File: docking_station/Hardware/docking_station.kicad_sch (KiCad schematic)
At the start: 26 parts, among them IC1 VOM1271T, IC2 VOM1271T, J1 SUPPLY_EN, J2 LIVE_IN, J5 SUPPLY+, J6 SUPPLY-, K1 Fujitsu_FTR-LYCA005x, K2 EC2-3NU, K3 EC2-3NU, Q1 NMOS, Q2 NMOS, Q3 NMOS, Q4 NMOS, Q5 NMOS, Q6 NMOS, Q7 NMOS, Q8 NMOS, Q9 NMOS, U1 LTC4357MS8

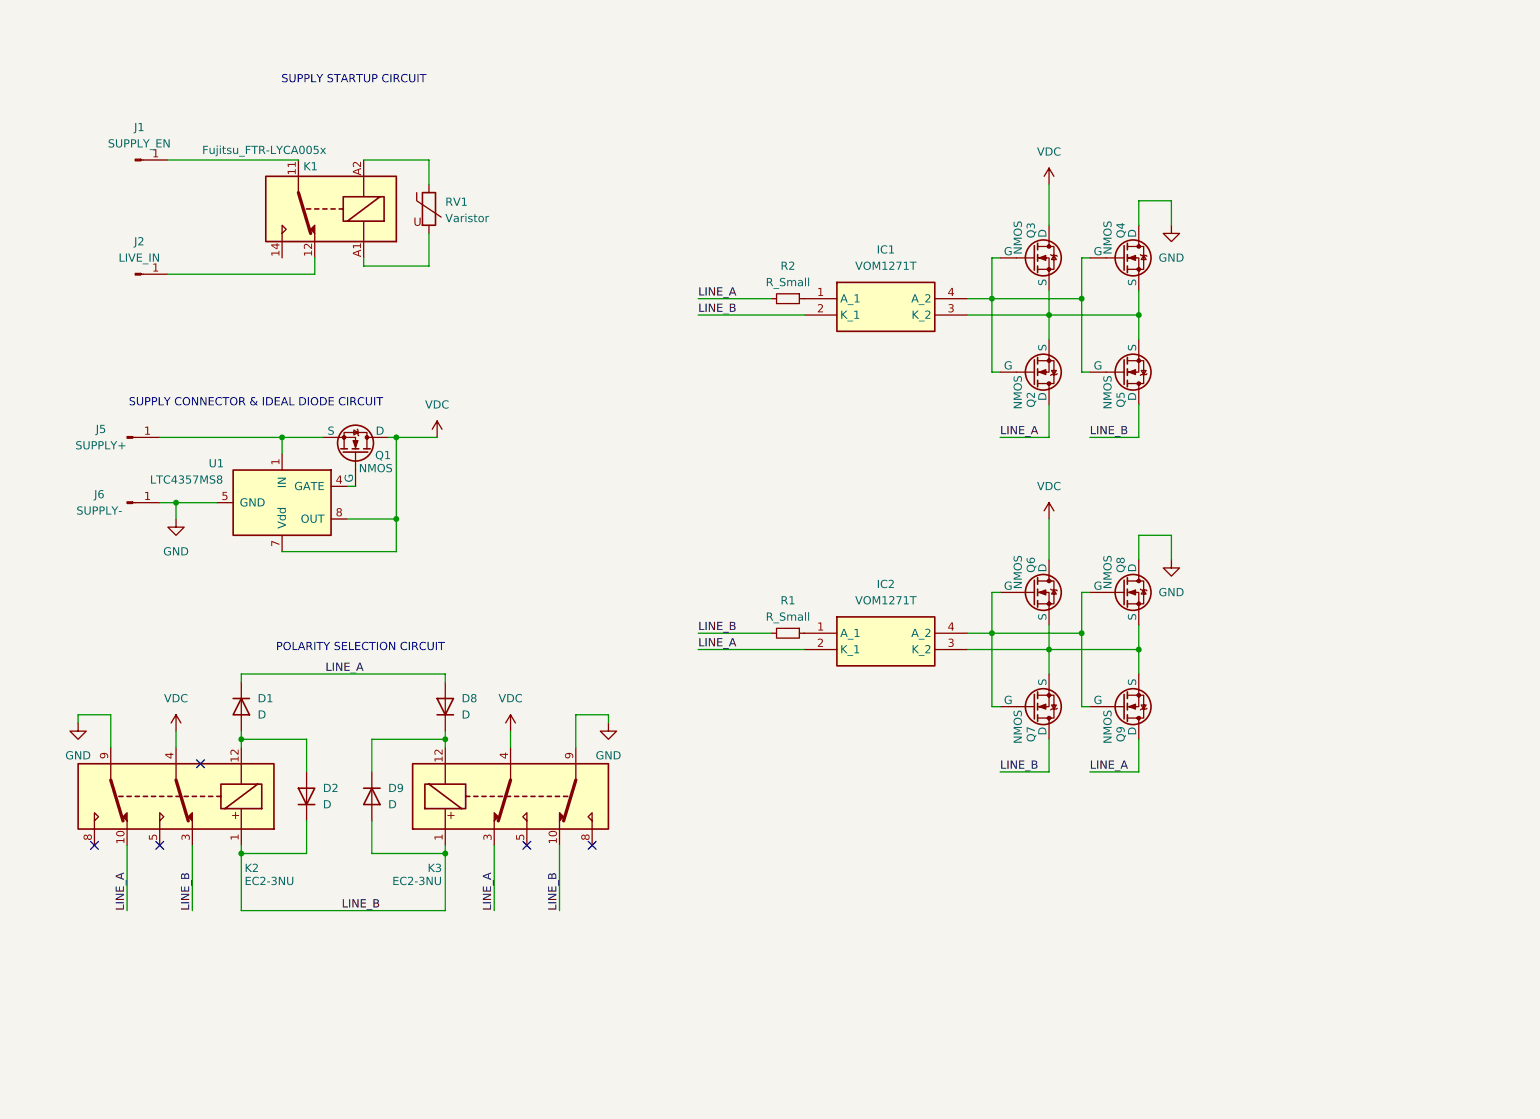
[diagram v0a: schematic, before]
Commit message: docking_station draft finished
a lot to do still - mostly calculation and review, but the bulk is done and I'm happy
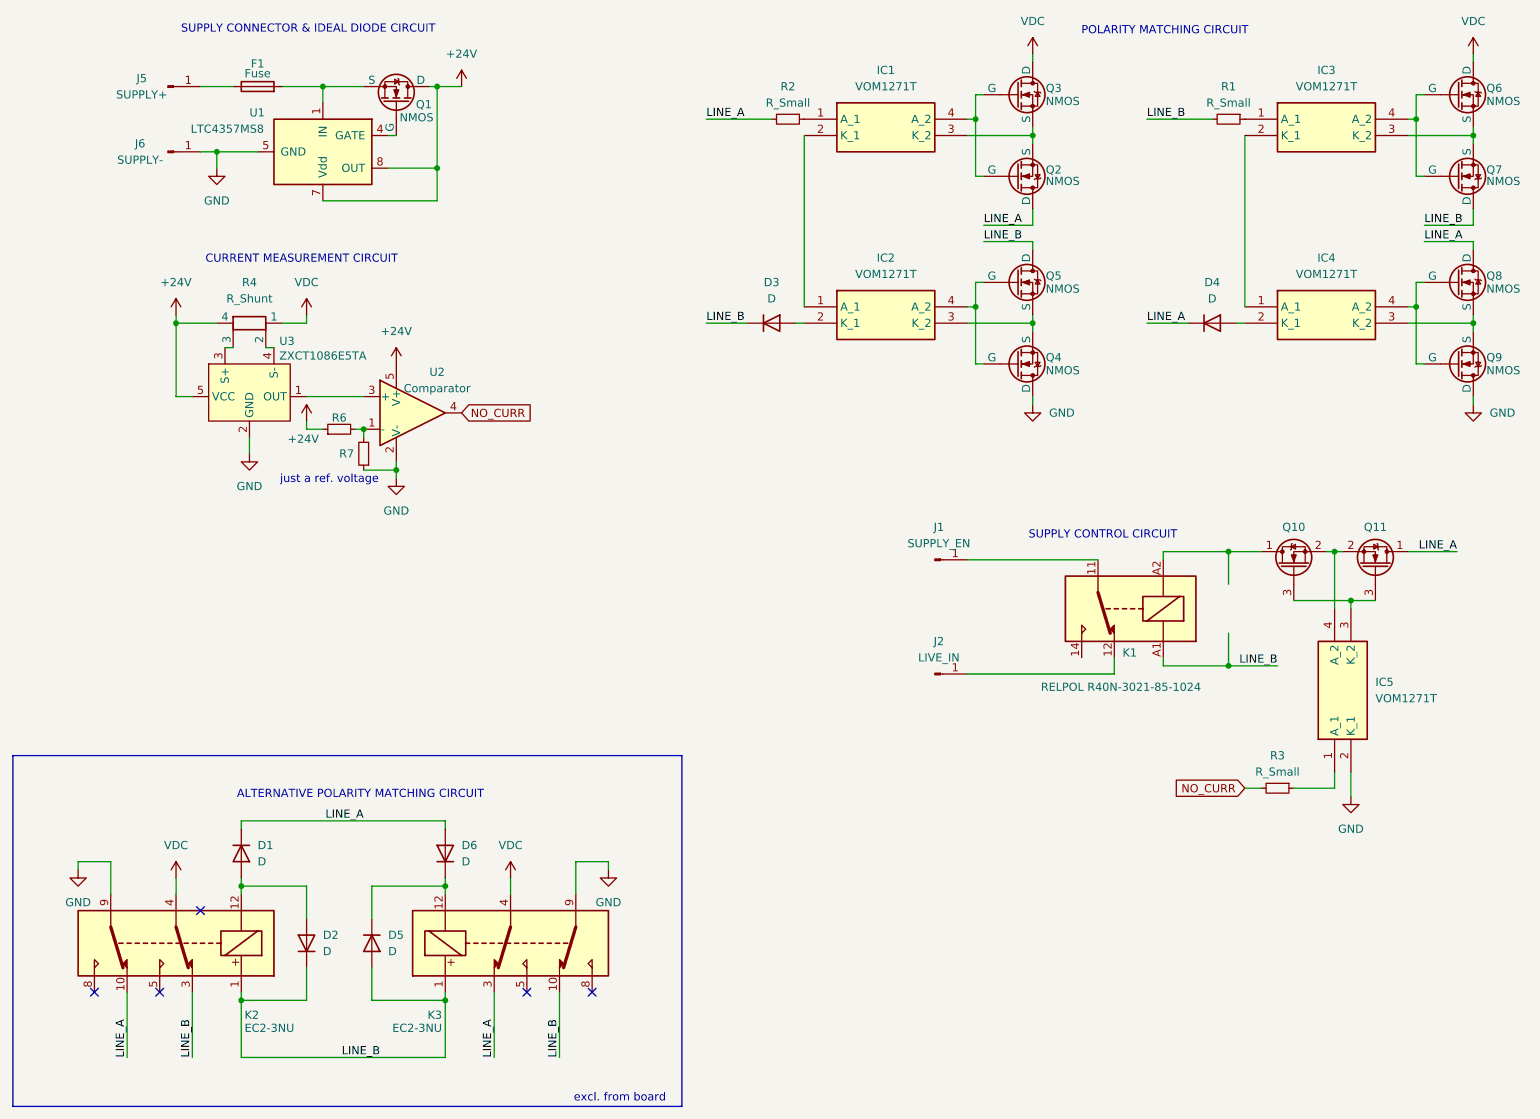
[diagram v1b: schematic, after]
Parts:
- removed D8, D9: D, symbol Device:D
- removed RV1: Varistor, symbol Device:Varistor
- added D3, D4, D5, D6: D, symbol Device:D
- added F1: Fuse, symbol Device:Fuse
- added IC3, IC4, IC5: VOM1271T, SOP254P675X240-4N, symbol VOM1271T:VOM1271T
- added Q10, Q11: Q_NMOS_Depletion_DSG, symbol Device:Q_NMOS_Depletion_DSG
- added R3, R6, R7: R_Small, symbol Device:R_Small
- added R4: R_Shunt, symbol Device:R_Shunt
- added U2: Comparator, Package_TO_SOT_SMD:SOT-23-5, symbol Comparator:LM397
- added U3: ZXCT1086E5TA, Package_TO_SOT_SMD:SOT-23-5, symbol FIRO_collected:ZXCT1086E5TA
- K1: value Fujitsu_FTR-LYCA005x -> RELPOL R40N-3021-85-1024
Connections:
- net GND: now also Q9.1 (D), IC5.2 (K_1), R7.1, U2.2 (V-), U3.2 (GND); no longer Q8.1 (D)
- net LINE_A: now also Q8.1 (D), D4.1 (K), D6.2 (A), Q11.1 (D); no longer IC2.2 (K_1), Q9.1 (D)
- net LINE_B: now also K1.A1, D3.1 (K), D5.2 (A); no longer IC1.2 (K_1)
- net VDC: now also R4.1; no longer Q1.1 (D), U1.7 (Vdd), U1.8 (OUT)
- net at K3.12: now also D5.1 (K), D6.1 (K)
- net at IC1.4 (A_2), Q2.2 (G), Q3.2 (G): no longer Q4.2 (G), Q5.2 (G)
- net at IC1.3 (K_2), Q2.3 (S), Q3.3 (S): no longer Q4.3 (S), Q5.3 (S)
- net at K1.A2: now also Q10.1 (D)
- net at Q1.3 (S), U1.1 (IN): now also F1.2; no longer J5.1 (Pin_1)
- net at R1.1: now also IC3.1 (A_1); no longer IC2.1 (A_1)
- new net: IC3.2 (K_1), IC4.1 (A_1)
- new net: IC3.3 (K_2), Q6.3 (S), Q7.3 (S)
- new net: IC3.4 (A_2), Q6.2 (G), Q7.2 (G)
- new net: F1.1, J5.1 (Pin_1)
- new net: IC5.4 (A_2), Q10.2 (S), Q11.2 (S)
- new net: IC5.3 (K_2), Q10.3 (G), Q11.3 (G)
- new net: IC5.1 (A_1), R3.1
- new net: IC4.4 (A_2), Q8.2 (G), Q9.2 (G)
- new net: IC4.3 (K_2), Q8.3 (S), Q9.3 (S)
- new net: R6.2, R7.2, U2.1 (-)
- new net: IC1.2 (K_1), IC2.1 (A_1)
- new net: IC2.4 (A_2), Q4.2 (G), Q5.2 (G)
- new net: IC2.3 (K_2), Q4.3 (S), Q5.3 (S)
- new net: D3.2 (A), IC2.2 (K_1)
- new net: U2.3 (+), U3.1 (OUT)
- new net: R4.3, U3.3 (S+)
- new net: R4.2, U3.4 (S-)
- new net: D4.2 (A), IC4.2 (K_1)
- new net +24V: Q1.1 (D), R4.4, R6.1, U1.7 (Vdd), U1.8 (OUT), U2.5 (V+), U3.5 (VCC)
- new net NO_CURR: R3.2, U2.4
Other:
- note added: "ALTERNATIVE POLARITY MATCHING CIRCUIT"
- note added: "CURRENT MEASUREMENT CIRCUIT"
- note added: "POLARITY MATCHING CIRCUIT"
- note added: "SUPPLY CONTROL CIRCUIT"
- note added: "excl. from board"
- note added: "just a ref. voltage"
- note removed: "POLARITY SELECTION CIRCUIT"
- note removed: "SUPPLY STARTUP CIRCUIT"
- moved on the sheet: IC1, J1, J2, J5, J6, K1, Q1, Q2, Q3, Q4, Q5, R2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
